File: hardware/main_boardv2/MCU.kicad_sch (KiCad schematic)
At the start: 5 parts, among them J301 Conn_01x03_Pin

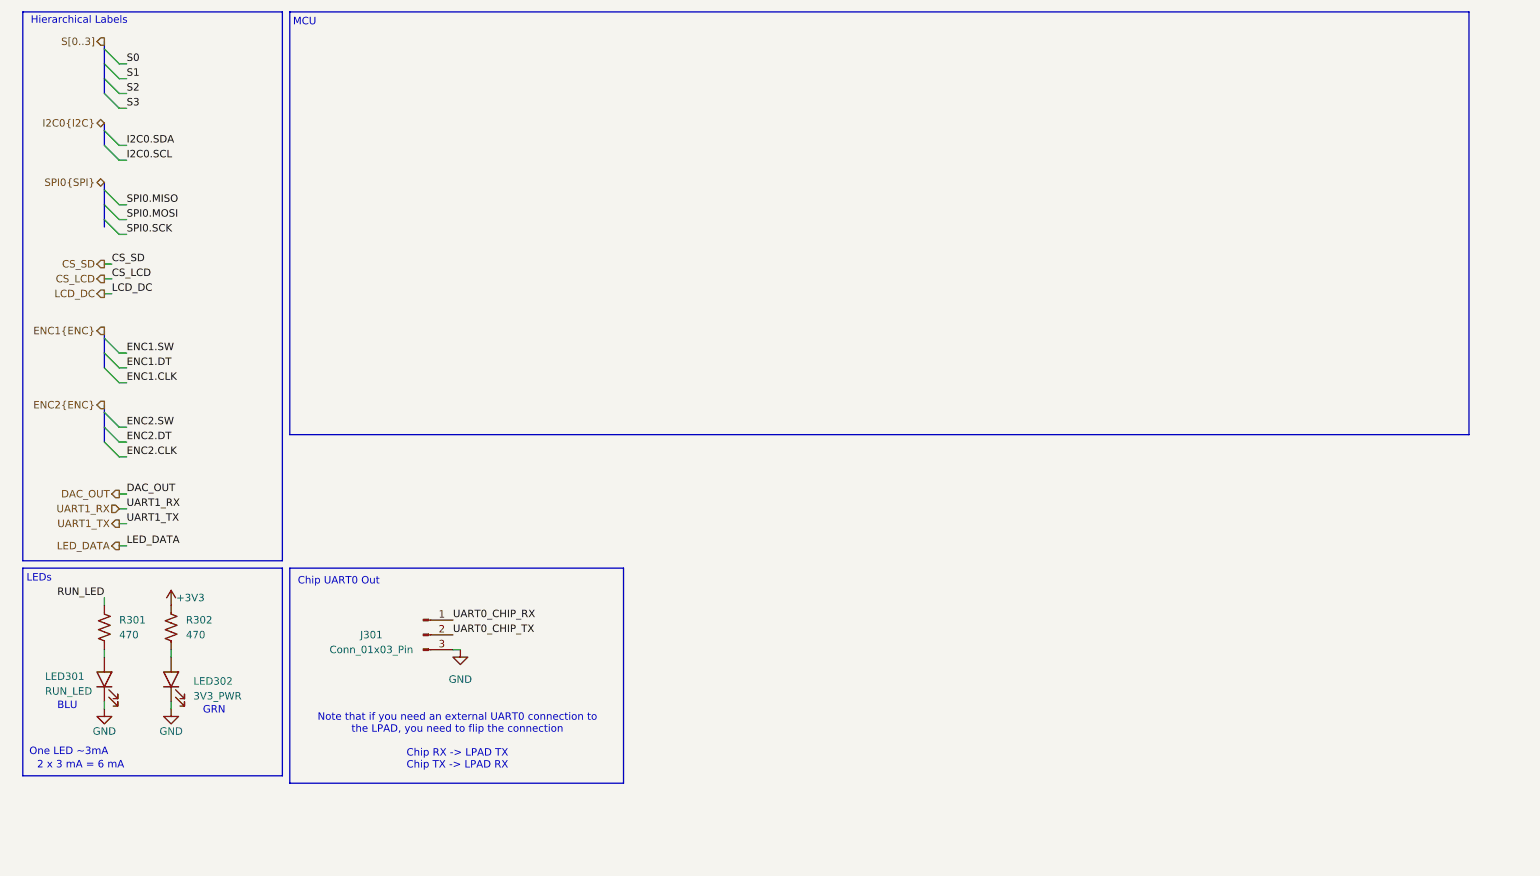
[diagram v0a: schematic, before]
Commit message: new hardware
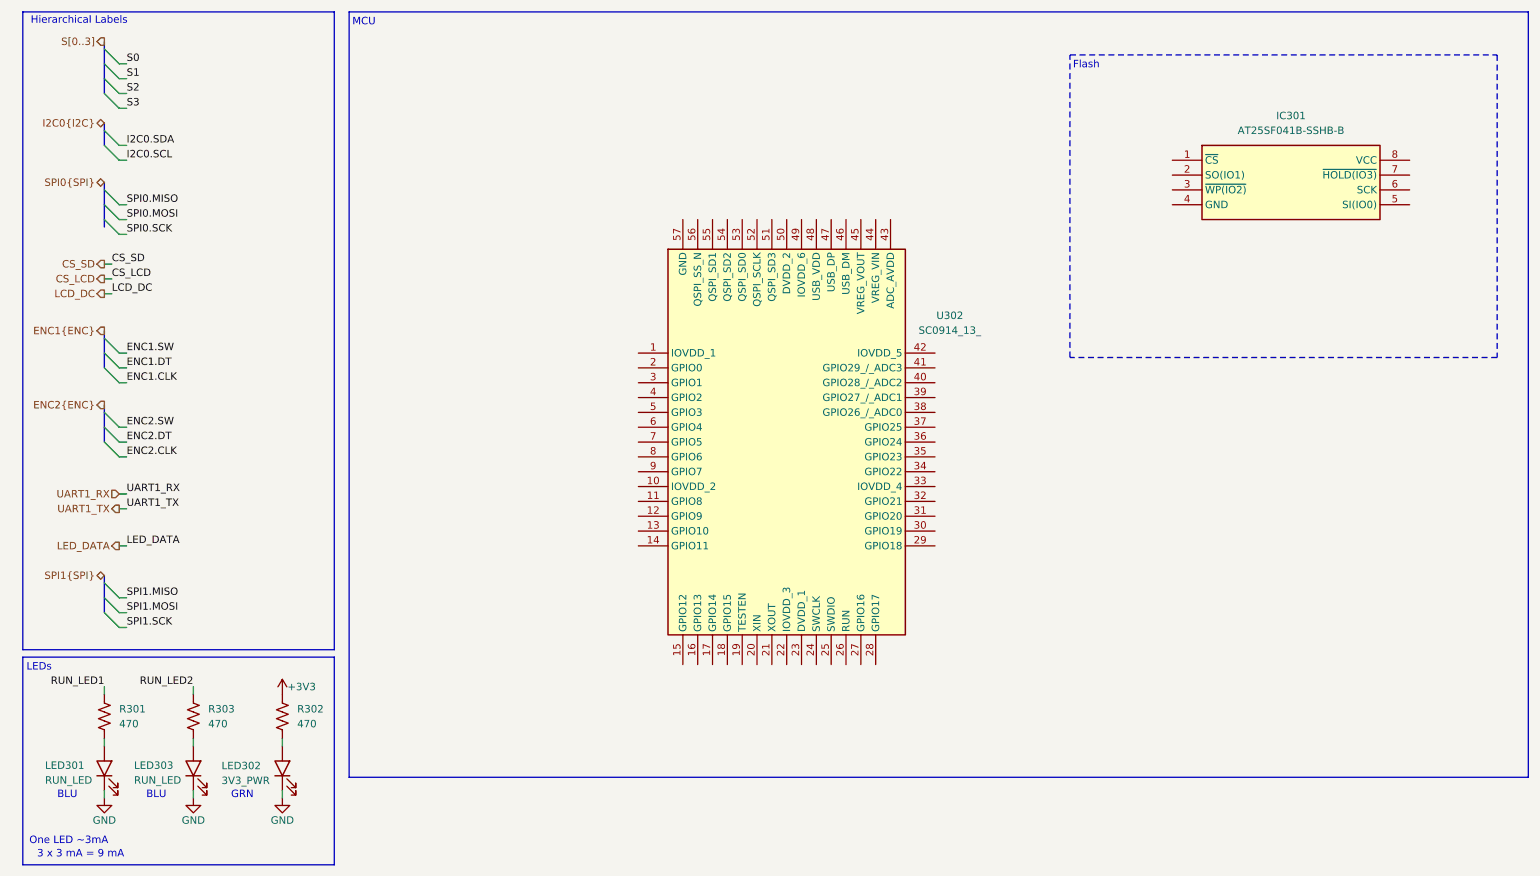
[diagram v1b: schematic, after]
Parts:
- removed J301: Conn_01x03_Pin, Connector_PinHeader_2.54mm:PinHeader_1x03_P2.54mm_Vertical, symbol Connector:Conn_01x03_Pin
- added IC301: AT25SF041B-SSHB-B, SOIC127P600X175-8N, symbol SamacSys_Parts:AT25SF041B-SSHB-B
- added LED303: RUN_LED, SamacSys_Parts:LEDC2012X40N, symbol ECE445L:LED
- added R303: 470, Resistor_SMD:R_0805_2012Metric, symbol Device:R_US
- added U302: SC0914_13_, SC091413, symbol SamacSys_Parts:SC0914_13_
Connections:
- net GND: now also LED303.1 (K)
- net RUN_LED renamed RUN_LED1
- new net: LED303.2 (A), R303.2
- new net RUN_LED2: R303.1
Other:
- note added: "3 x 3 mA = 9 mA"
- note added: "Flash"
- note removed: "2 x 3 mA = 6 mA"
- note removed: "Chip UART0 Out"
- note removed: "Note that if you need an external UART0 connection to the LPAD, you need to flip the connection Chip RX -> LPAD TX Chip TX -> LPAD RX"
- moved on the sheet: LED301, LED302, R301, R302
